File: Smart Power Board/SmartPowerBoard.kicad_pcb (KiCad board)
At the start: 4 copper layers, 41.8 x 41.5 mm, 94 parts, among them J1 430450200, J2 USB_C_Receptacle_USB2.0_16P, J3 430450200, J4 Conn_01x02_Socket, J5 Screw_Terminal_01x02, J6 Screw_Terminal_01x02, Q1 PMOS, Q2 NMOS, SW1 SW_Push, SW2 SW_Push, SW3 SW_Push, U1 INA3221, U2 X096-2864TMBAG01-H30, U4 TPS56C230RJER, U5 TPS56C230RJER, U6 RP2040, U7 W25Q32JVSS, Y1 FL1200138

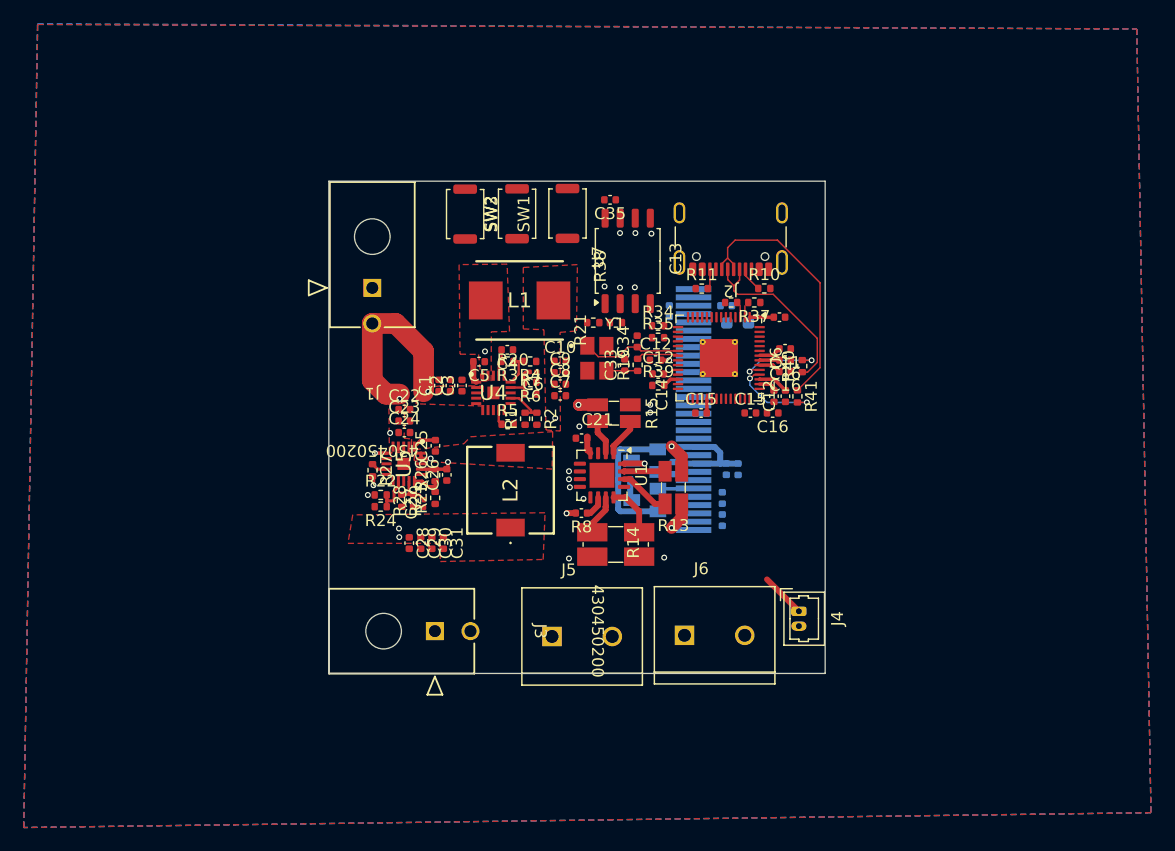
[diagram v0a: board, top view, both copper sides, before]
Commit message: Feat[SmartPowerBoard]: New Layout
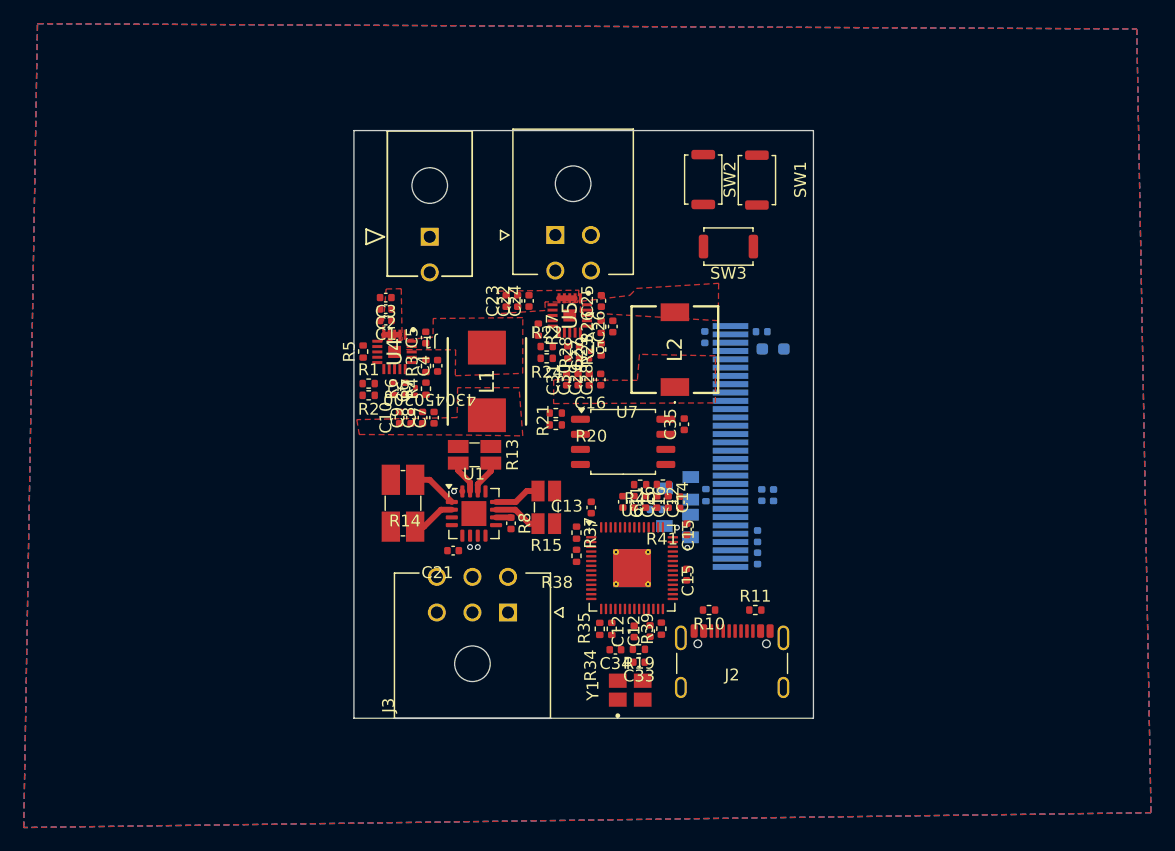
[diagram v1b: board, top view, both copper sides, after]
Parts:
- removed J4: Conn_01x02_Socket, Connector_Molex:Molex_PicoBlade_53047-0210_1x02_P1.25mm_Vertical
- removed J6: Screw_Terminal_01x02, 282837_2:TE_282837-2
- J3: value 430450200 -> 430450601; footprint ul_430450200:CON_430450200_MOL -> 430450601:MOLEX_430450601
- J5: value Screw_Terminal_01x02 -> 430450400; footprint 282837_2:TE_282837-2 -> 430450400:MOLEX_430450400
- moved J2 37.8 mm to (169.2, 122.0), turned to 0 degrees
- moved J5 33.9 mm to (154.2, 85.0), turned to 180 degrees
- moved Y1 28.1 mm to (160.6, 123.3), turned to 90 degrees
- moved R10 27.5 mm to (167.2, 116.6), turned to 180 degrees
- moved R11 27.5 mm to (171.1, 116.6)
- moved C34 26.1 mm to (159.3, 119.9), turned to 180 degrees
- moved R34 26.0 mm to (158.0, 118.2), turned to 90 degrees
- moved C33 25.1 mm to (161.3, 121.0), turned to 180 degrees
- moved R38 25.0 mm to (156.0, 112.0), turned to 90 degrees
- moved R35 24.8 mm to (159.0, 118.2), turned to 90 degrees
- moved R37 24.5 mm to (156.0, 110.0), turned to -90 degrees
- moved R19 24.0 mm to (161.3, 119.9), turned to 180 degrees
- moved C12 22.9 mm to (160.9, 118.4), turned to 90 degrees
- moved C13 22.6 mm to (157.3, 107.9), turned to -90 degrees
- moved SW3 22.4 mm to (168.8, 85.9), turned to 180 degrees
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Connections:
- J1 pad 1: GND -> unconnected-(J1-Pad1)
- J3 pad 2: /Triple Channel Monitor/12V_{OUT} -> GND
- J5 pad 2: /Triple Channel Monitor/5V_{OUT} -> GND
- R13 pad 4: /Buck Converter 5V/V_{OUT} -> /Triple Channel Monitor/5V_{IN}
- R14 pad 1: /12V_{IN} -> /Triple Channel Monitor/12V_{IN}
- R14 pad 2: Net-(U1-IN-1) -> Net-(U1-IN-3)
- R14 pad 3: Net-(U1-IN+1) -> Net-(U1-IN+3)
- R15 pad 2: Net-(U1-IN-3) -> Net-(U1-IN-1)
- R15 pad 3: Net-(U1-IN+3) -> Net-(U1-IN+1)
- R27 pad 2: Net-(U5-VCC) -> /Buck Converter 3.3V/V_{CC}
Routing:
- net /12V_{IN}: track 53.8 -> 0.00 mm, vias 3 -> 0
- net /3.3V_{IN}: track 23.3 -> 0.00 mm, vias 2 -> 0
- net /MCU/USB_M: track 22.6 -> 0.00 mm
- net /Triple Channel Monitor/3.3V_{IN}: track 21.9 -> 0.00 mm, vias 3 -> 0
- net /Triple Channel Monitor/12V_{OUT}: track 20.8 -> 0.00 mm, vias 1 -> 0
- net /Triple Channel Monitor/5V_{OUT}: track 19.0 -> 0.00 mm, vias 1 -> 0
- net /MCU/USB_P: track 15.9 -> 0.00 mm
- net /Buck Converter 5V/V_{OUT}: track 13.5 -> 0.00 mm, vias 2 -> 0
- net /Triple Channel Monitor/3.3V: track 13.5 -> 0.02 mm, vias 3 -> 1
- net /MCU/3.3V: track 12.9 -> 0.00 mm, vias 1 -> 0
- net Net-(Q1-G): track 11.7 -> 0.00 mm
- net Net-(U5-VCC): track 10.7 -> 0.00 mm, vias 2 -> 0
- net /MCU/XIN: track 8.49 -> 0.00 mm
- net Net-(U6-USB_DM): track 7.72 -> 0.00 mm, vias 2 -> 0
- net Net-(U6-USB_DP): track 7.31 -> 0.00 mm, vias 2 -> 0
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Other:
- board size 41.8 x 41.5 mm -> 38.7 x 49.5 mm
- board text added: "YOU CAN CHANGE THIS"
